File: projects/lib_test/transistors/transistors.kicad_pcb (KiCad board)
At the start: 2 copper layers, 43 x 21 mm, 11 parts, among them Q1 MMBT2222A, Q10 MJL3281A, Q11 MJL1302A, Q2 AO3400A, Q3 DMP3028LFDE, Q4 CEM3083, Q5 VBZA4800, Q6 BC850B, Q7 BC860B, Q8 BD139, Q9 BD140

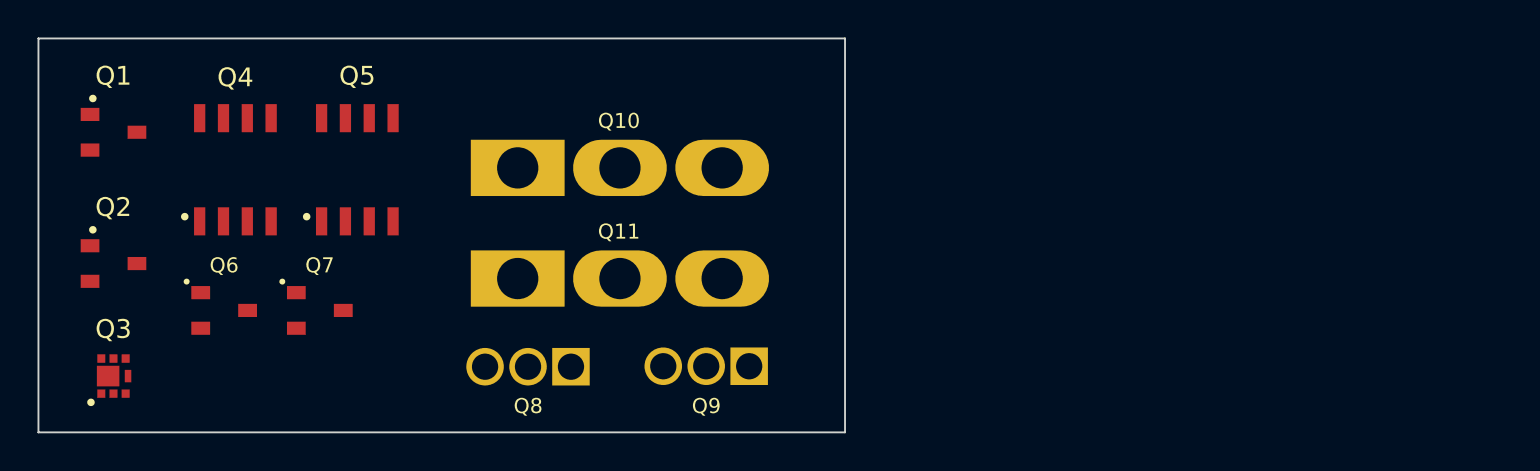
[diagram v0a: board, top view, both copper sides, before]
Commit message: updated transistors test project
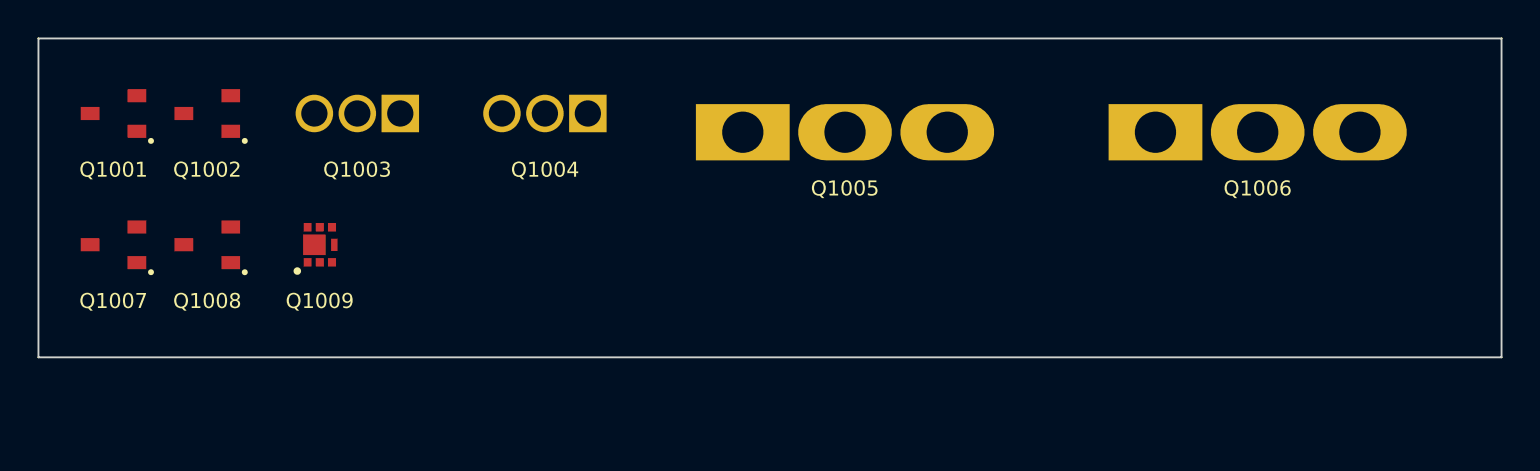
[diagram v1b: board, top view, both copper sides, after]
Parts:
- removed Q1: MMBT2222A, lily_footprints:sot23
- removed Q2: AO3400A, lily_footprints:sot23
- removed Q4: CEM3083, lily_footprints:soic8
- removed Q5: VBZA4800, lily_footprints:soic8
- added Q1007: MMBT2222AL, lily_footprints:sot23, F.Cu at (114.0, 81.0)
- added Q1008: DMG3406L, lily_footprints:sot23, F.Cu at (119.0, 81.0)
- moved Q1006 34.9 mm to (169.6, 75.0)
- moved Q1003 16.3 mm to (124.7, 74.0)
- moved Q1004 16.0 mm to (134.7, 74.0)
- moved Q1009 13.0 mm to (125.0, 81.0)
- moved Q1005 12.1 mm to (147.6, 75.0)
- moved Q1002 12.1 mm to (119.0, 74.0), turned to 0 degrees
- moved Q1001 12.0 mm to (114.0, 74.0), turned to 0 degrees
- renumbered Q6 to Q1001, Q7 to Q1002, Q8 to Q1003, Q9 to Q1004, Q10 to Q1005, Q11 to Q1006, Q3 to Q1009
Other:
- board size 43 x 21 mm -> 78 x 17 mm
